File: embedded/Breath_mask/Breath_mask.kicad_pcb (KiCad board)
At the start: 2 copper layers, 38 parts, among them IC1 TPS61291DRVR, J2 USB, J4 Conn_ST_STDC14, SW2 SW_Push, SW3 SW_Push, U1 LPS22HBTR, U23 M95256, U4 STM32L052K8Tx

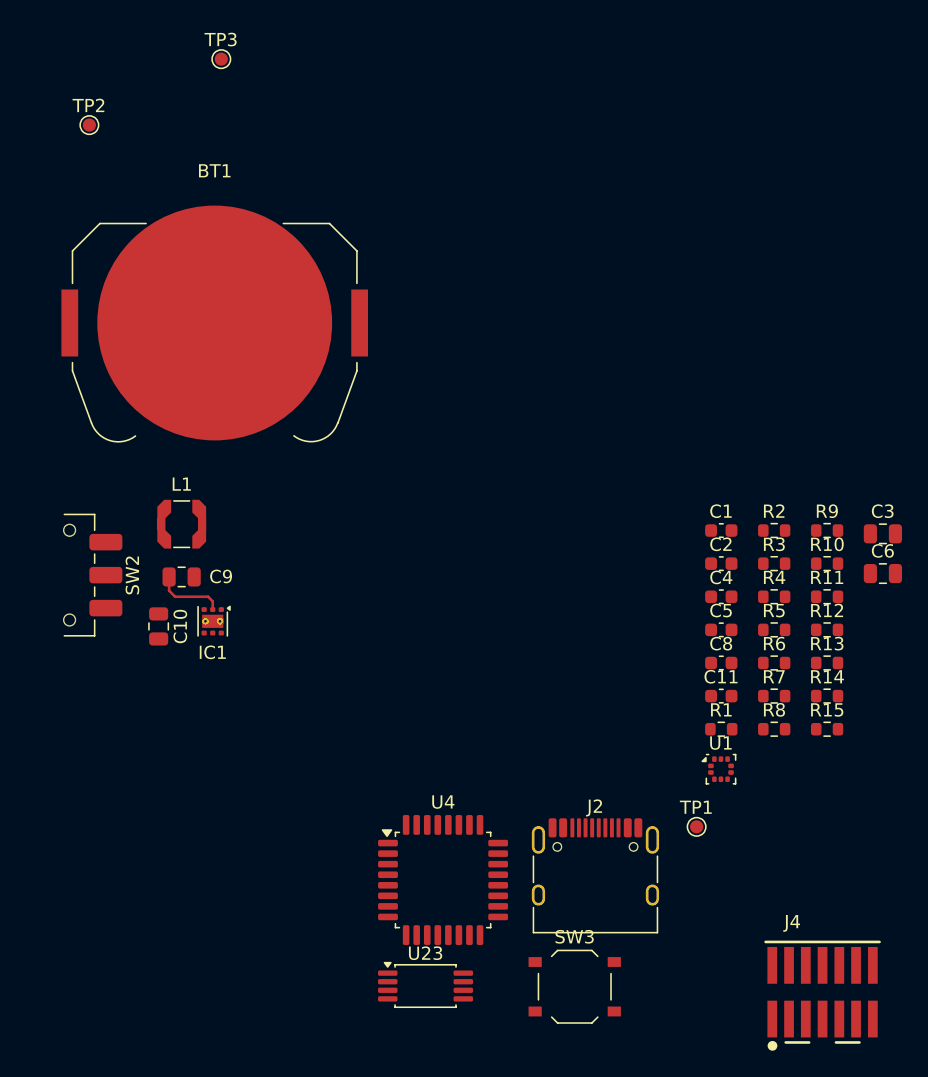
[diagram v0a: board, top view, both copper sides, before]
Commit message: Aggiornamento sbroglio
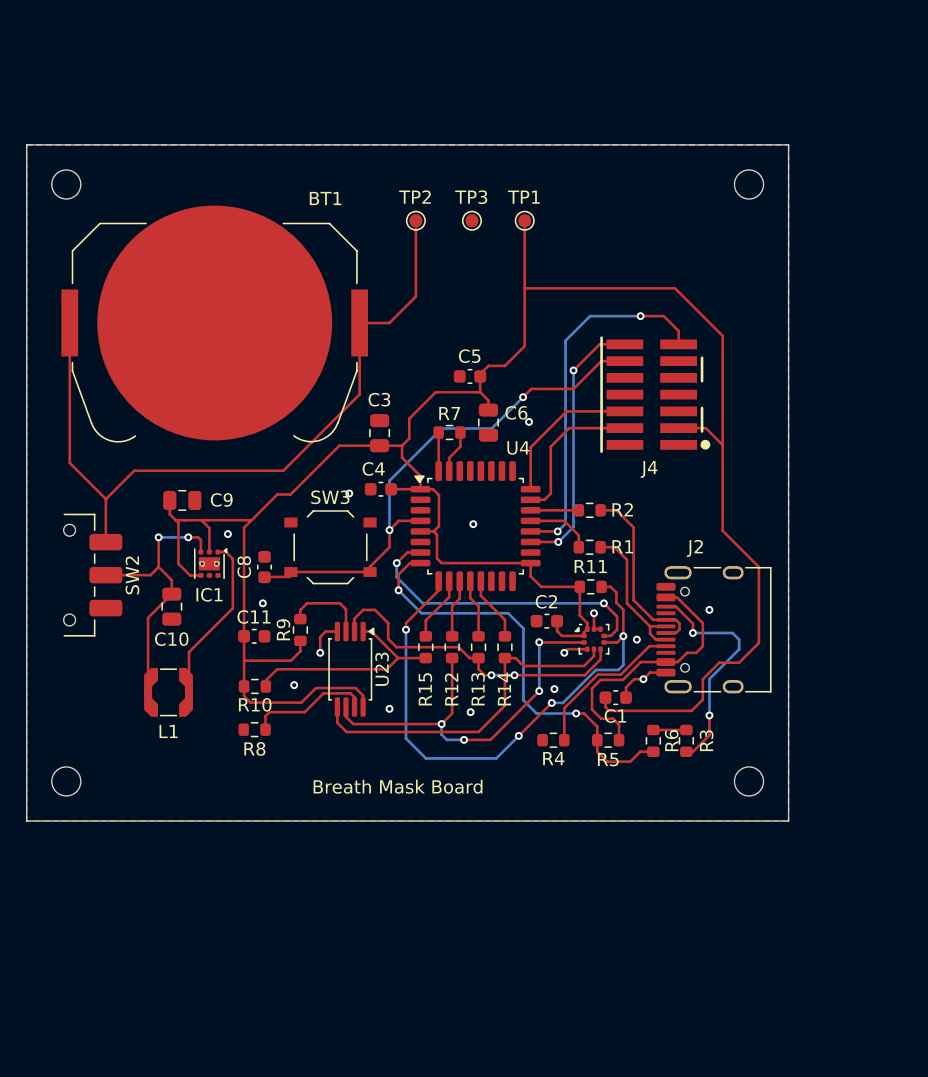
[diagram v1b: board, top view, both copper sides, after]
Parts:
- added G***: LOGO, LOGO, B.Cu at (115.8, 87.8)
- moved TP1 47.8 mm to (137.5, 48.2)
- moved J4 47.1 mm to (147.1, 61.4), turned to 90 degrees
- moved R10 44.4 mm to (117.0, 83.5), turned to 180 degrees
- moved R9 40.6 mm to (120.5, 79.3), turned to -90 degrees
- moved R8 39.4 mm to (117.0, 86.8)
- moved C3 38.9 mm to (126.5, 64.3), turned to -90 degrees
- moved SW3 38.1 mm to (122.8, 73.0)
- moved C11 35.7 mm to (117.0, 79.8)
- moved C8 35.4 mm to (117.8, 74.5), turned to -90 degrees
- moved C6 32.0 mm to (134.8, 63.5), turned to 90 degrees
- moved R7 31.7 mm to (131.8, 64.3)
- moved R15 31.0 mm to (130.0, 80.6), turned to -90 degrees
- moved R12 28.5 mm to (132.0, 80.6), turned to -90 degrees
- moved C4 27.1 mm to (126.6, 68.6)
- moved C5 27.1 mm to (133.3, 60.0)
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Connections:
- SW2 pad 3: (no net) -> GND
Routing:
- net +3V3: track 5.31 -> 178.0 mm
- net Net-(BT1-+): track 0.00 -> 56.5 mm
- net /SENS_CS: track 0.00 -> 41.9 mm, vias 0 -> 4
- net /~{RST}: track 0.00 -> 40.1 mm, vias 0 -> 2
- net /USB_F: track 0.00 -> 32.5 mm, vias 0 -> 2
- net /SPI1_SCK: track 0.00 -> 30.6 mm, vias 0 -> 4
- net /USART1_RX: track 0.00 -> 27.6 mm, vias 0 -> 2
- net /SPI1_MOSI: track 0.00 -> 26.4 mm
- net /SPI1_MISO: track 0.00 -> 24.4 mm, vias 0 -> 2
- net /INTERRUPT_SENS: track 0.00 -> 23.3 mm, vias 0 -> 2
- net Net-(IC1-VIN): track 0.00 -> 21.4 mm, vias 0 -> 2
- net Net-(J2-VBUS-PadA4): track 0.00 -> 20.4 mm
- net /USART1_TX: track 0.00 -> 20.3 mm, vias 0 -> 2
- net Net-(J2-CC2): track 0.00 -> 17.4 mm, vias 0 -> 2
- net /MEM_CS: track 0.00 -> 16.8 mm
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- added copper zone on B.Cu, net GND
- added copper zone on F.Cu, net GND
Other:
- board outline added: 57.8 x 51.2 mm
- board text added: "Anna Dal Mas, Alessia Rinaldi"
- board text added: "Breath Mask Board"
- board text added: "Low-Power Embedded Systems Project"
